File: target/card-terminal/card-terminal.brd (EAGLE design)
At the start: 77 x 70.8 mm, 33 parts, among them IC1 74S113D, Q1 16 MHz, Q2 BSS123, Q3 BSS123, Q4 BSS123, Q5 BSS123, Q6 BSS123, X2 5036-008-210-862

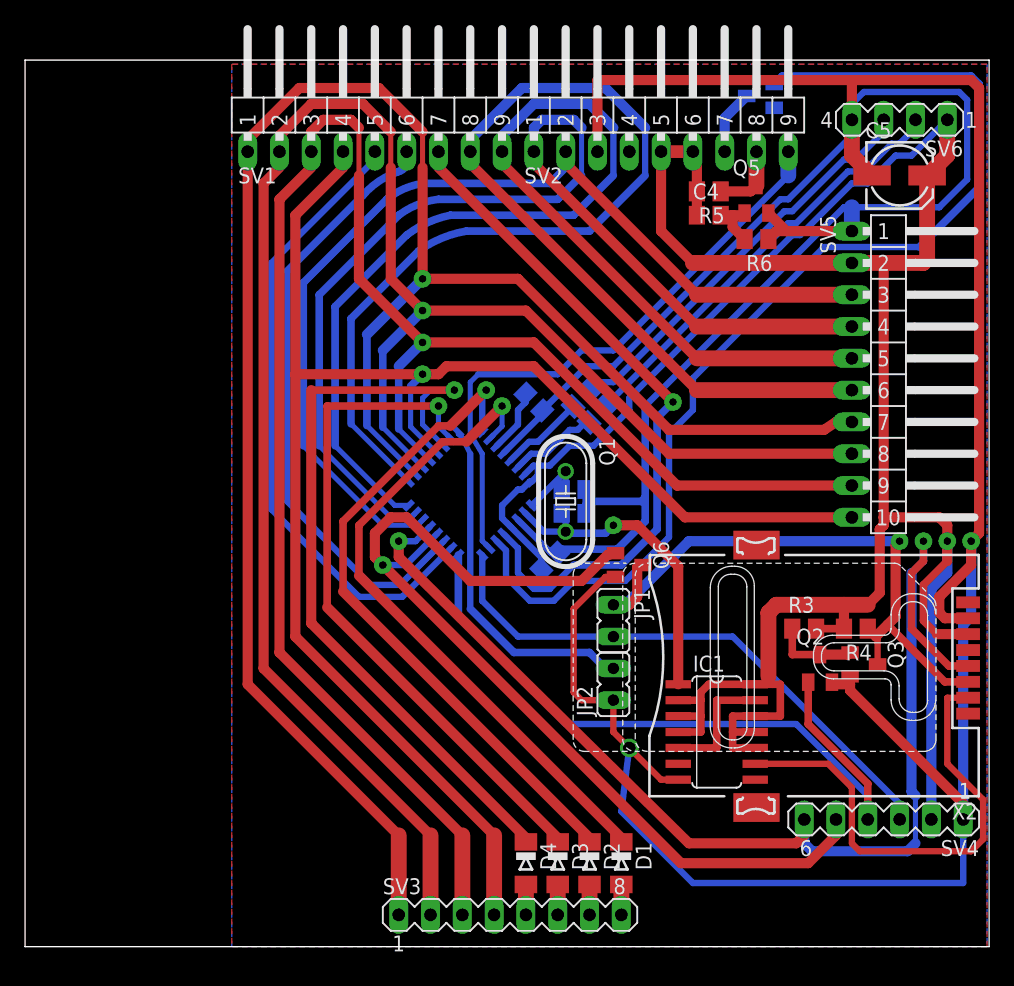
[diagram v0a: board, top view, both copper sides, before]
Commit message: fixes for card-terminal hardware
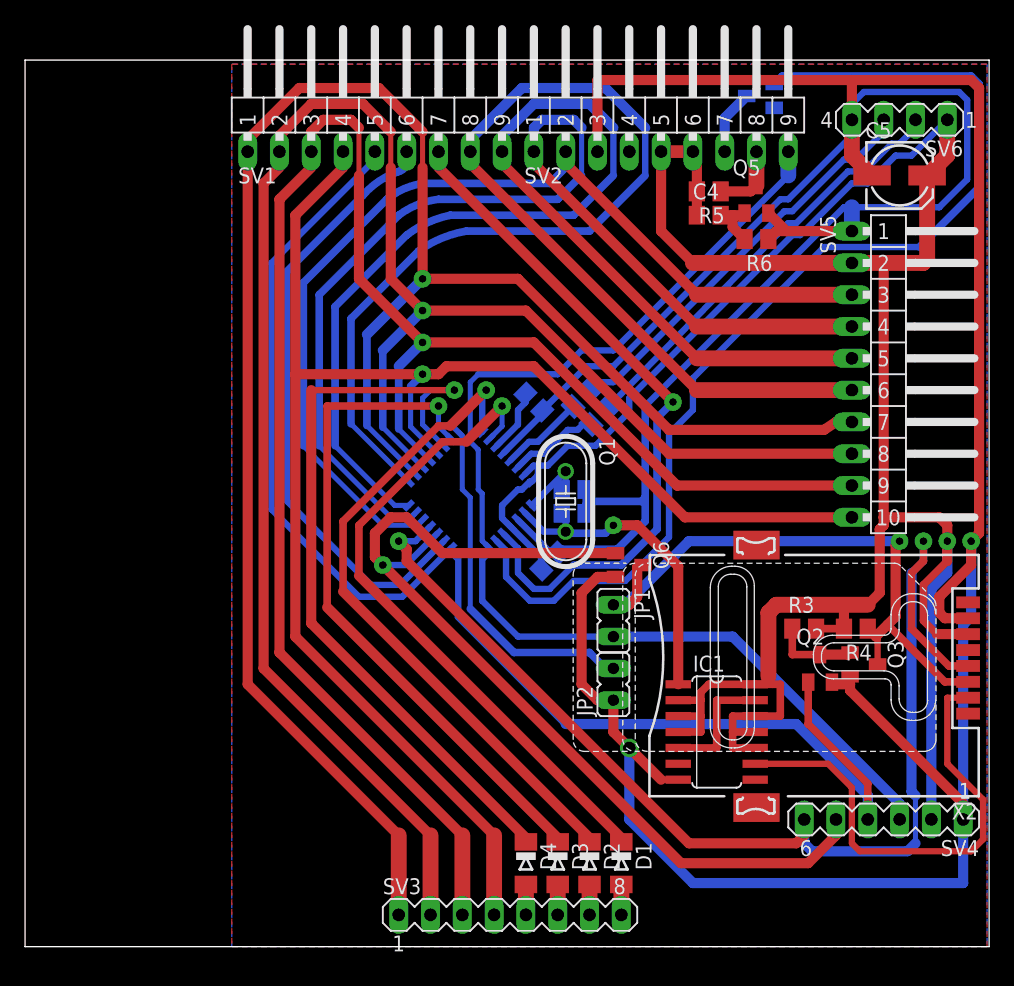
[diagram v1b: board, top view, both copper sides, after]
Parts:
- moved R2 0.22 mm to (45.9, 42.4)
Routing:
- net GND: track 324.0 -> 322.1 mm
- net RTS: track 79.1 -> 77.4 mm
